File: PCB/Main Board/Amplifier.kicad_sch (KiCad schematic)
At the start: 30 parts

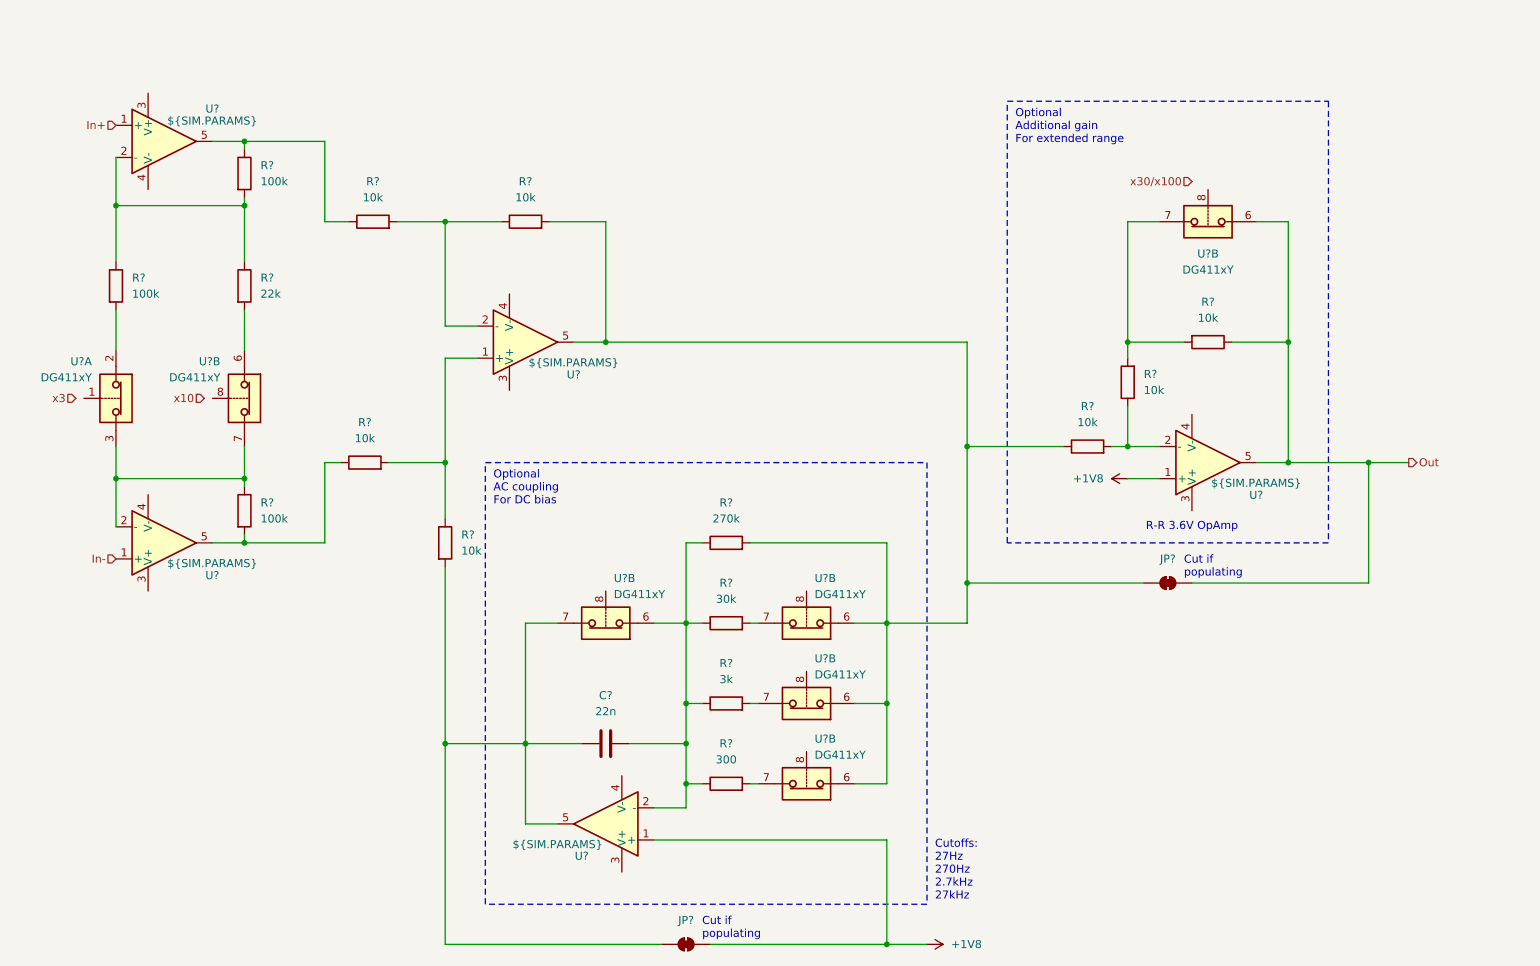
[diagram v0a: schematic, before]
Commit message: InAmp Progress
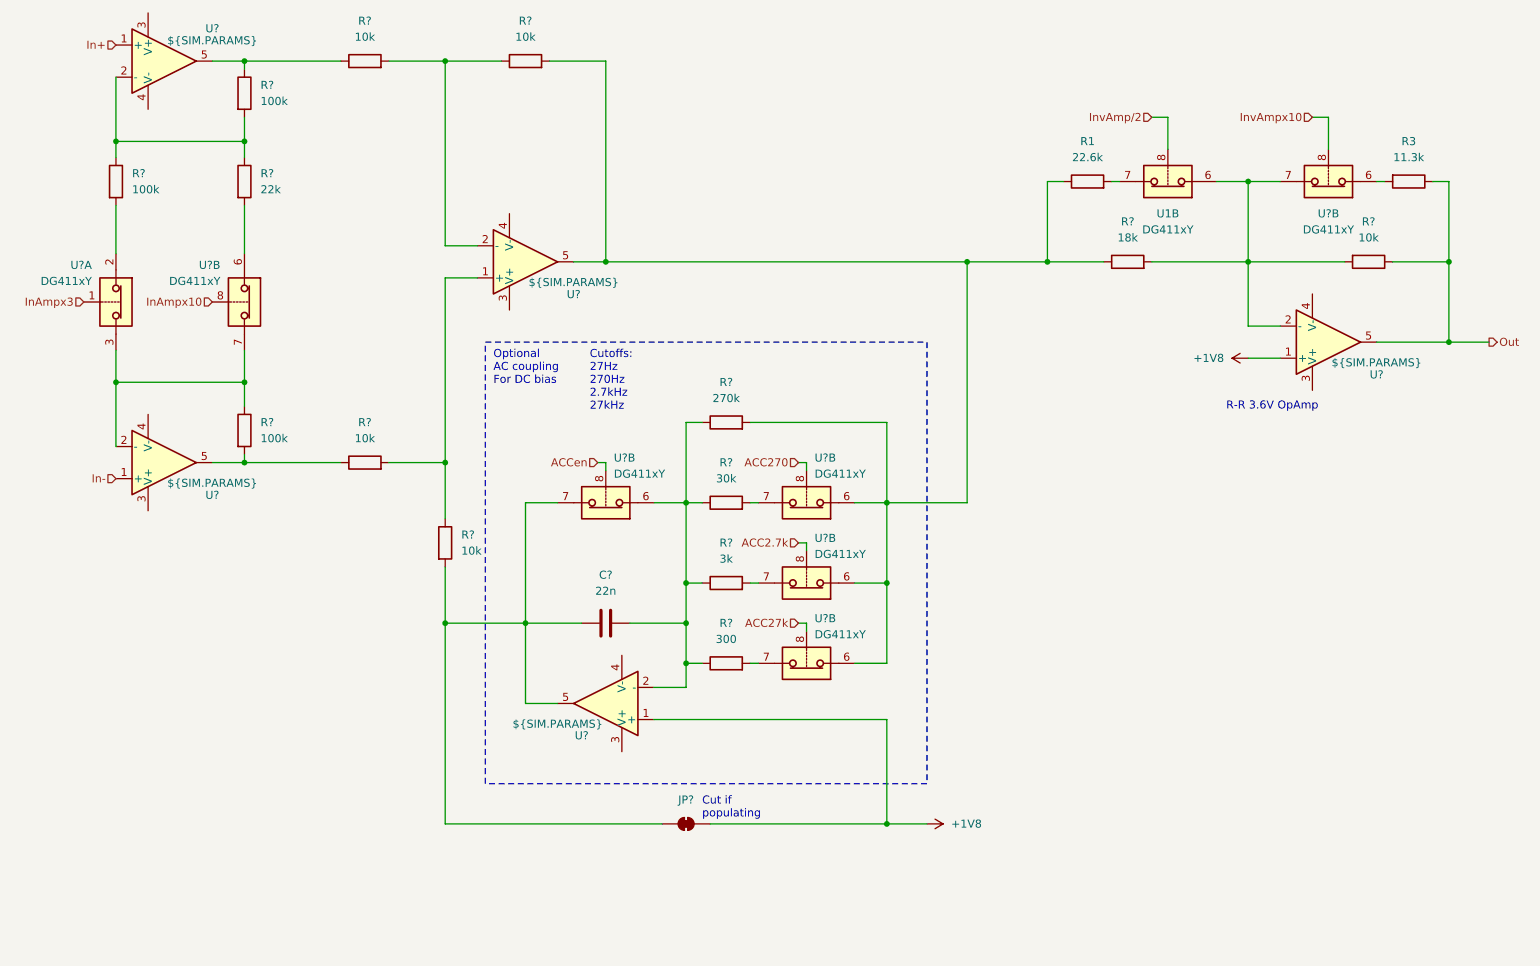
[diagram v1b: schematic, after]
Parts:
- removed JP?: SolderJumper_2_Bridged, Jumper:SolderJumper-2_P1.3mm_Bridged_RoundedPad1.0x1.5mm, symbol Jumper:SolderJumper_2_Bridged
- removed R?: 10k, symbol Device:R
- added R1: 22.6k, symbol Device:R
- added R3: 11.3k, symbol Device:R
- added U1: DG411xY, Package_SO:SOIC-16_3.9x9.9mm_P1.27mm, symbol Analog_Switch:DG411xY
- R?: value 10k -> 18k
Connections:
- net Out: now also R3.1; no longer U?.6
- net at R?.2, U?.7: now also R?.2, U?.2 (-), U1.6
- net InvAmpx10: now reaches U?.8
- net at R?.1, R?.2, R?.2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: now also R1.1
- net ACC27k: now reaches U?.8
- net ACC270: now reaches U?.8
- net InAmpx10: now reaches U?.8
- net ACCen: now reaches U?.8
- net ACC2.7k: now reaches U?.8
- net InAmpx3: now reaches U?.1
- new net: R1.2, U1.7
- new net: R3.2, U?.6
- new net InvAmp/2: U1.8
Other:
- note removed: "Optional Additional gain For extended range"
- company: (none) -> Harry and Yuki - EEE3 Instrumentation
- title: (none) -> Instrumentation Amplifier
- moved on the sheet: C?, JP?, R?, U?, U?A, U?B
